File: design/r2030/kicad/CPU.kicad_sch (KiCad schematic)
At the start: 13 parts, among them IC1 MC68030RC_PGA, IC8 ATF16V8BQL, Q2 5H8ET-20.000

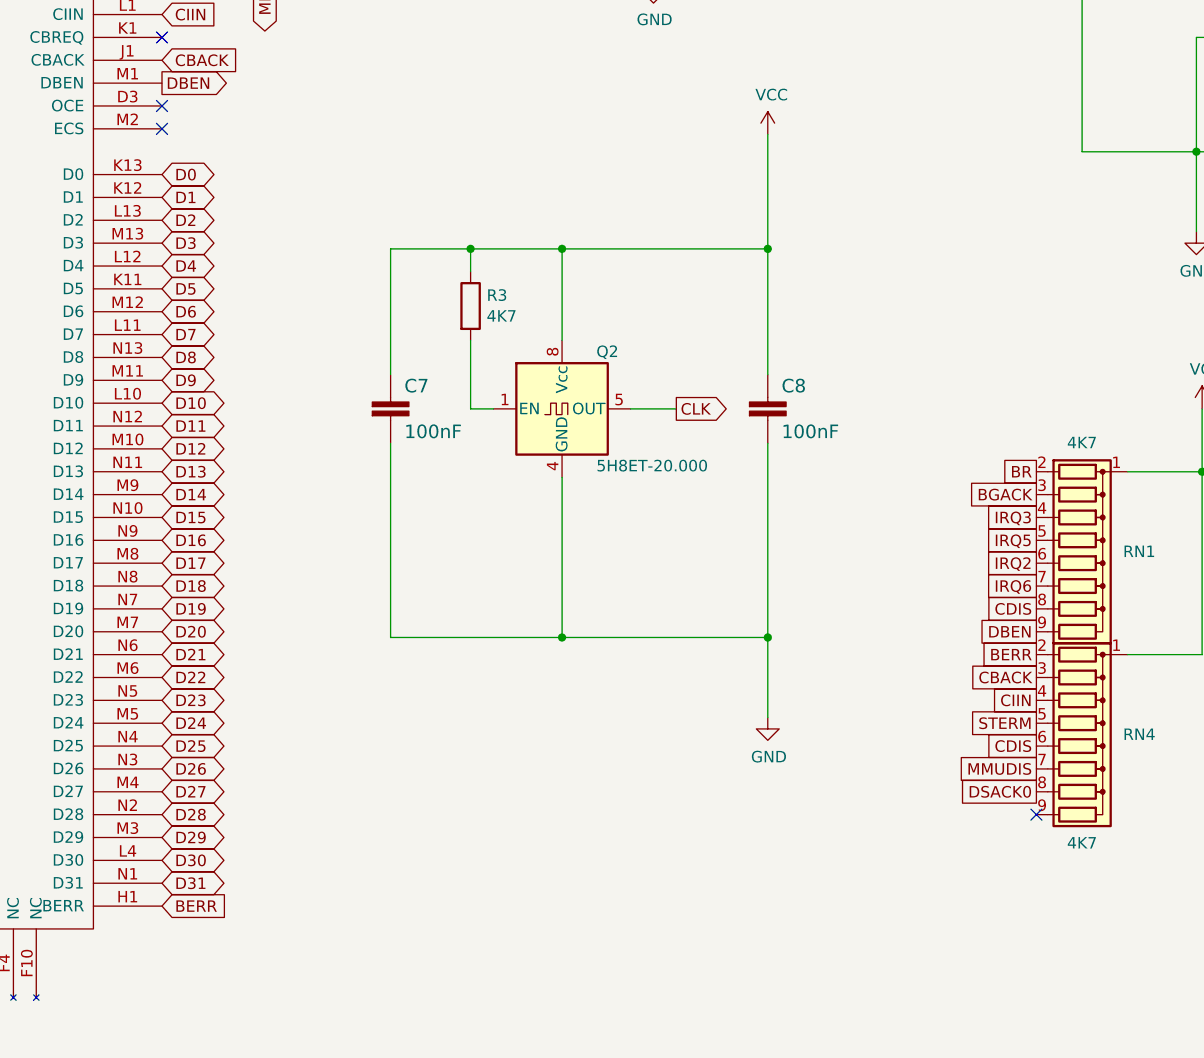
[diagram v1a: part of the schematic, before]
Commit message: Fix pre-prod bugs
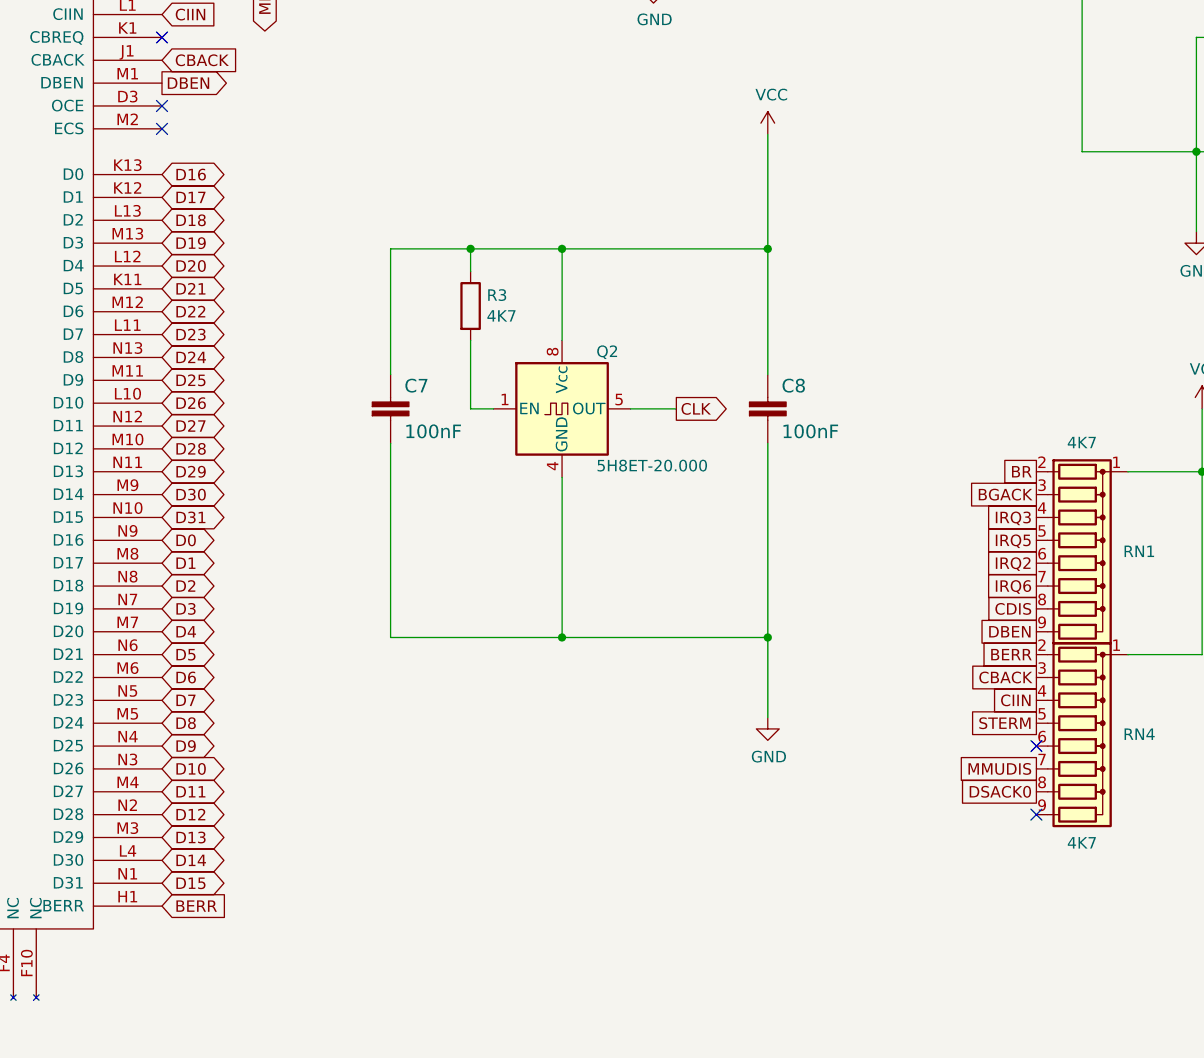
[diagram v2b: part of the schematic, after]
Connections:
- net CDIS: no longer RN4.6 (R5)
- net D0: now also IC1.N9 (D16); no longer IC1.K13 (D0)
- net D1: now also IC1.M8 (D17); no longer IC1.K12 (D1)
- net D10: now also IC1.N3 (D26); no longer IC1.L10 (D10)
- net D11: now also IC1.M4 (D27); no longer IC1.N12 (D11)
- net D12: now also IC1.N2 (D28); no longer IC1.M10 (D12)
- net D13: now also IC1.M3 (D29); no longer IC1.N11 (D13)
- net D14: now also IC1.L4 (D30); no longer IC1.M9 (D14)
- net D15: now also IC1.N1 (D31); no longer IC1.N10 (D15)
- net D16: now also IC1.K13 (D0); no longer IC1.N9 (D16)
- net D17: now also IC1.K12 (D1); no longer IC1.M8 (D17)
- net D18: now also IC1.L13 (D2); no longer IC1.N8 (D18)
- net D19: now also IC1.M13 (D3); no longer IC1.N7 (D19)
- net D2: now also IC1.N8 (D18); no longer IC1.L13 (D2)
- net D20: now also IC1.L12 (D4); no longer IC1.M7 (D20)
- net D21: now also IC1.K11 (D5); no longer IC1.N6 (D21)
- net D22: now also IC1.M12 (D6); no longer IC1.M6 (D22)
- net D23: now also IC1.L11 (D7); no longer IC1.N5 (D23)
- net D24: now also IC1.N13 (D8); no longer IC1.M5 (D24)
- net D25: now also IC1.M11 (D9); no longer IC1.N4 (D25)
- net D26: now also IC1.L10 (D10); no longer IC1.N3 (D26)
- net D27: now also IC1.N12 (D11); no longer IC1.M4 (D27)
- net D28: now also IC1.M10 (D12); no longer IC1.N2 (D28)
- net D29: now also IC1.N11 (D13); no longer IC1.M3 (D29)
- net D3: now also IC1.N7 (D19); no longer IC1.M13 (D3)
- net D30: now also IC1.M9 (D14); no longer IC1.L4 (D30)
- net D31: now also IC1.N10 (D15); no longer IC1.N1 (D31)
- net D4: now also IC1.M7 (D20); no longer IC1.L12 (D4)
- net D5: now also IC1.N6 (D21); no longer IC1.K11 (D5)
- net D6: now also IC1.M6 (D22); no longer IC1.M12 (D6)
- net D7: now also IC1.N5 (D23); no longer IC1.L11 (D7)
- net D8: now also IC1.M5 (D24); no longer IC1.N13 (D8)
- net D9: now also IC1.N4 (D25); no longer IC1.M11 (D9)
- no-connect marks 25 -> 26

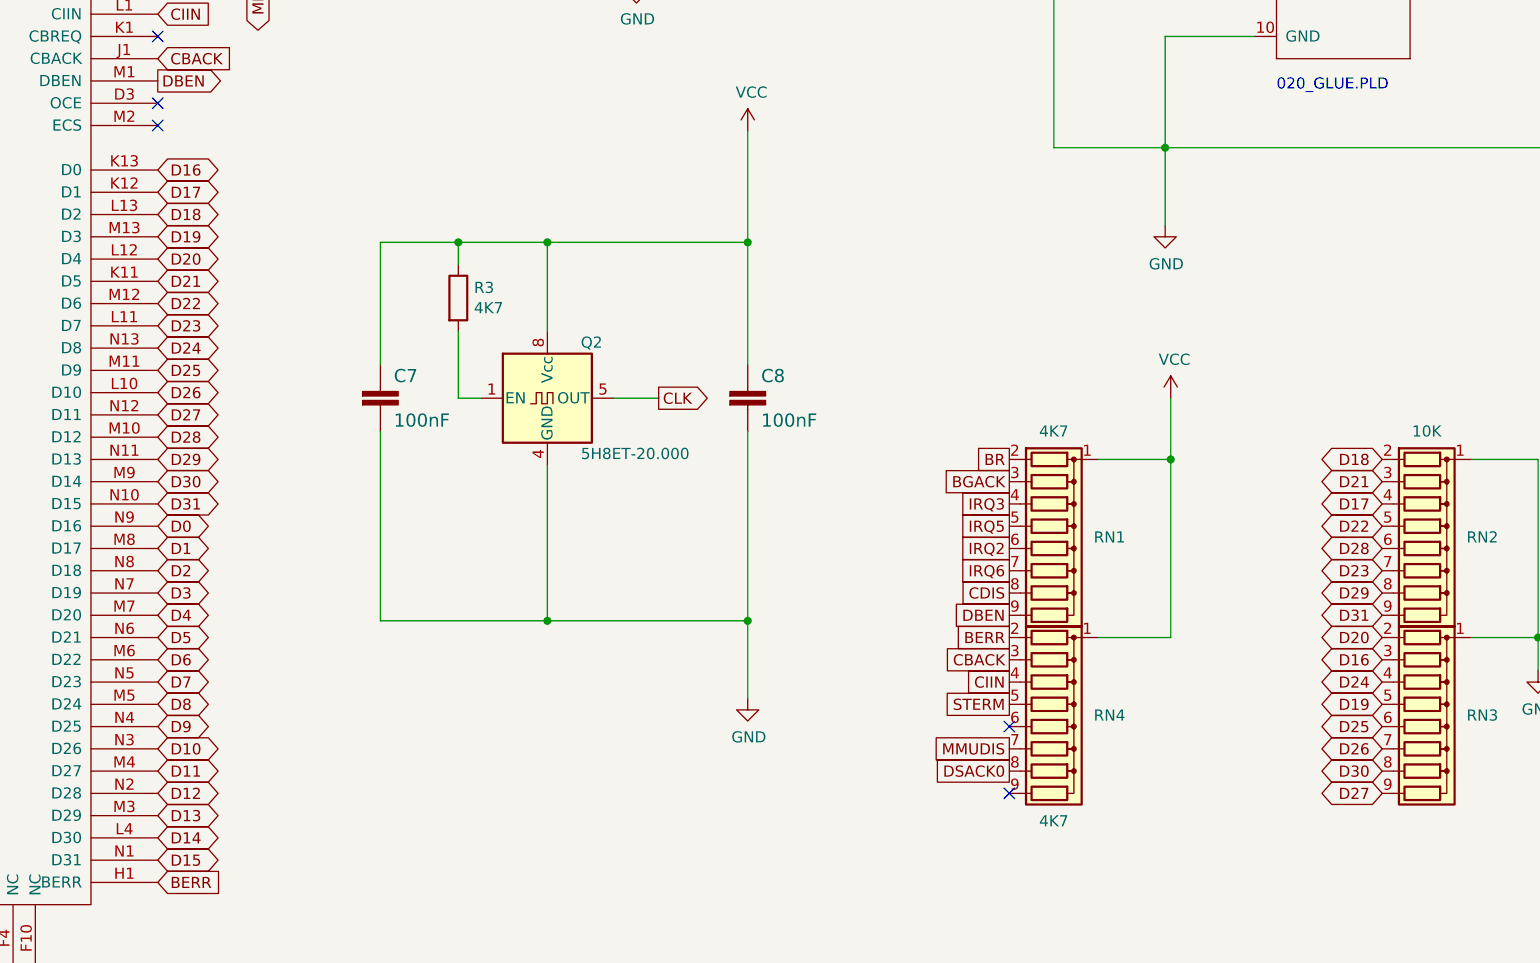
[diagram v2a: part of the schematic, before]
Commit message: Cleanup
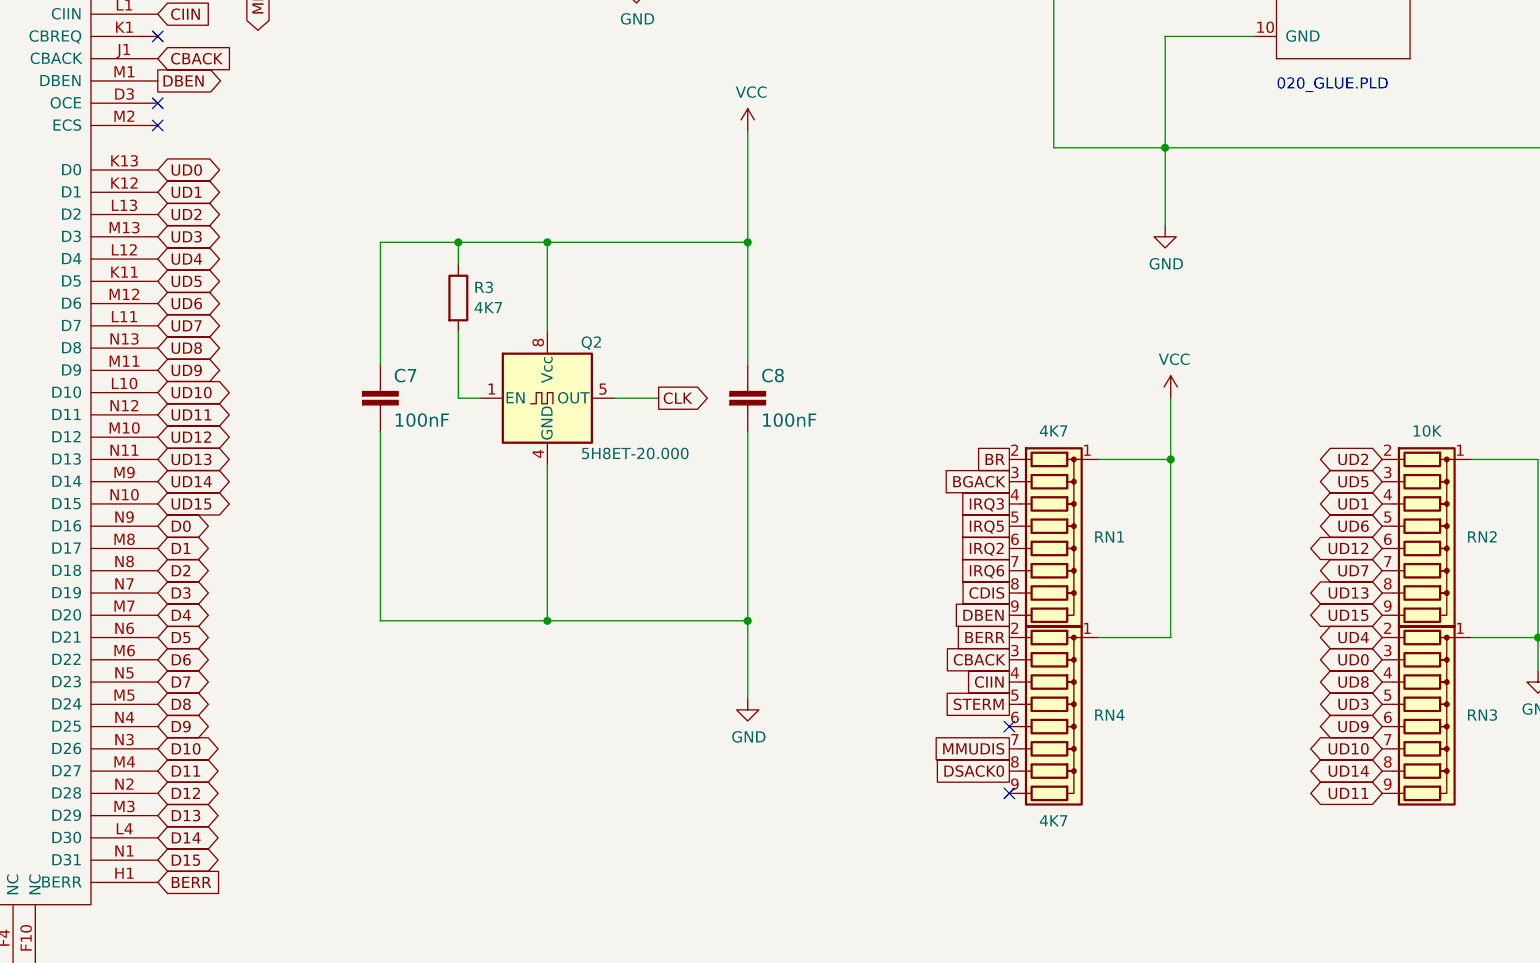
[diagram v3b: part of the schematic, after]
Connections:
- net D16 renamed UD0
- net D17 renamed UD1
- net D18 renamed UD2
- net D19 renamed UD3
- net D20 renamed UD4
- net D21 renamed UD5
- net D22 renamed UD6
- net D23 renamed UD7
- net D24 renamed UD8
- net D25 renamed UD9
- net D26 renamed UD10
- net D27 renamed UD11
- net D28 renamed UD12
- net D29 renamed UD13
- net D30 renamed UD14
- net D31 renamed UD15
